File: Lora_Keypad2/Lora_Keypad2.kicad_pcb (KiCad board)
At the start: 2 copper layers, 53.3 x 76.2 mm, 7 parts, among them J1 OLED Conn

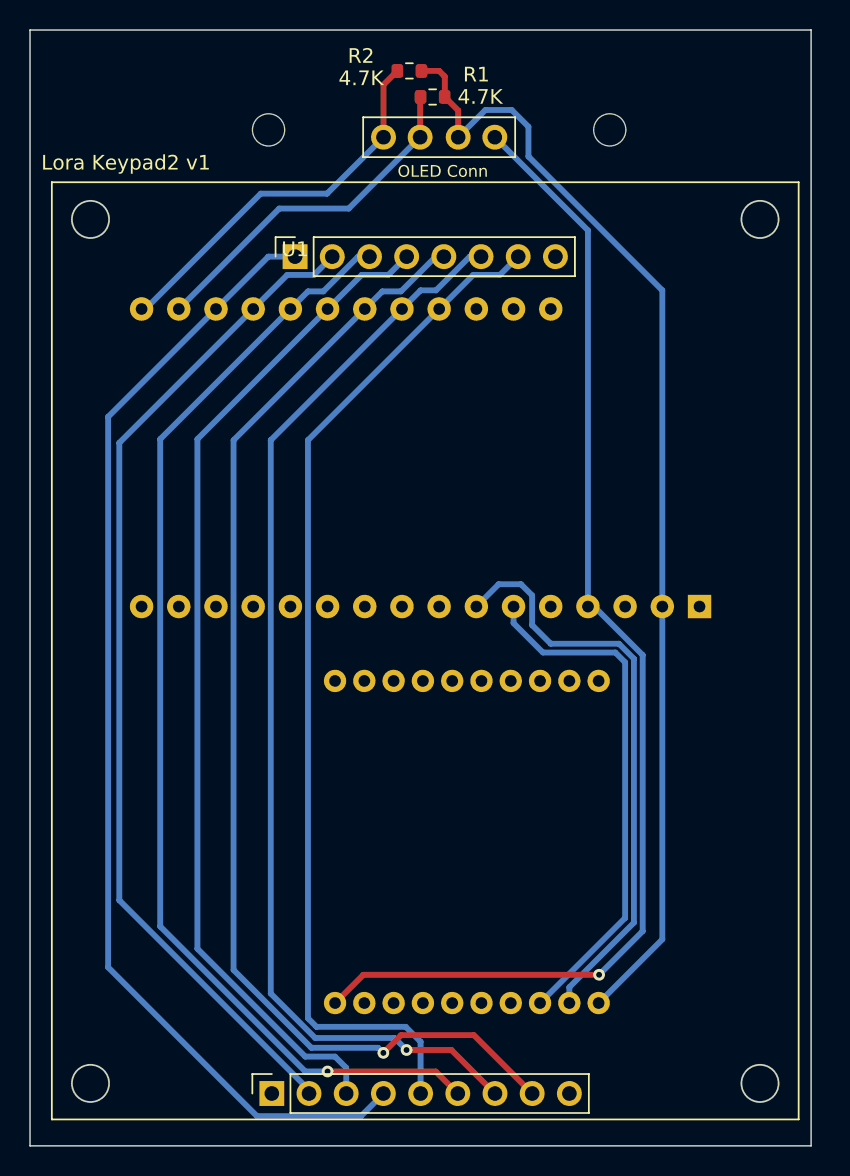
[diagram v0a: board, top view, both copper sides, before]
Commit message: update
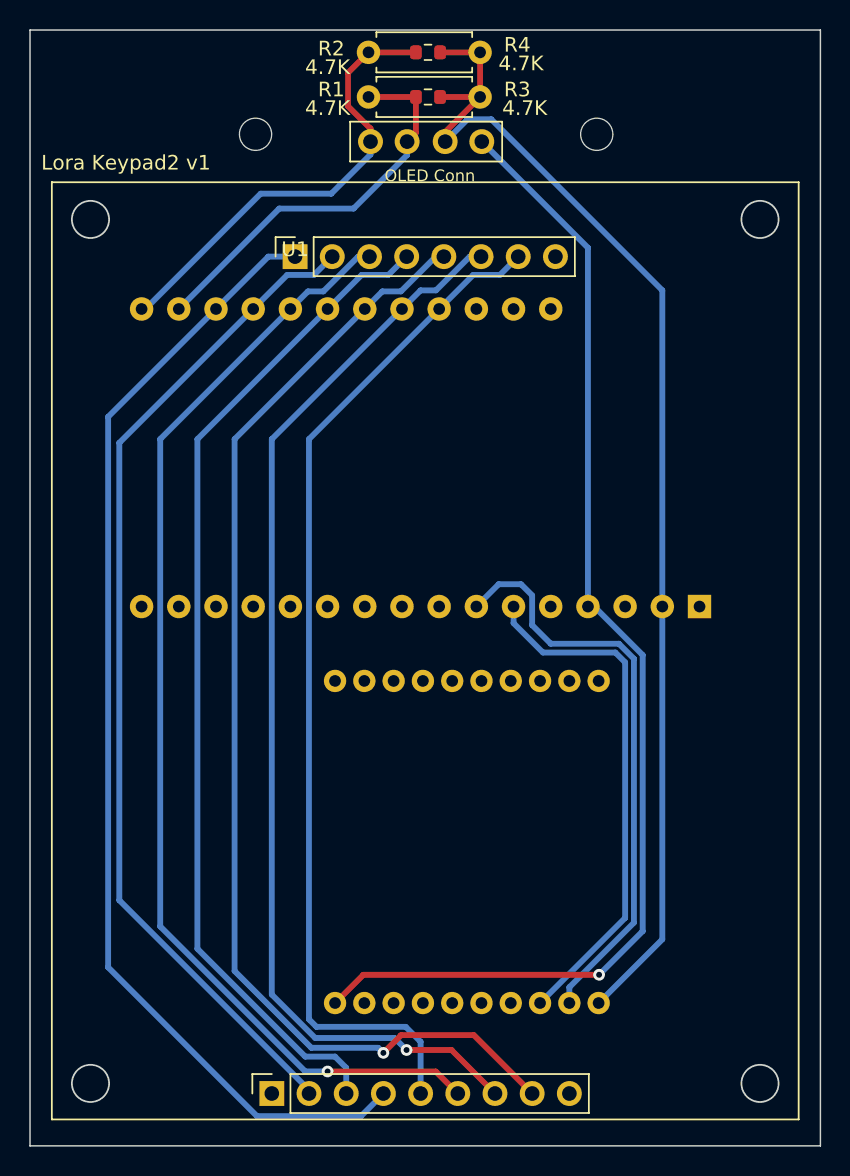
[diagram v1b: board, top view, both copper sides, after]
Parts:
- added R3: 4.7K, Resistor_THT:R_Axial_DIN0207_L6.3mm_D2.5mm_P7.62mm_Horizontal, F.Cu at (203.5, 60.5)
- added R4: 4.7K, Resistor_THT:R_Axial_DIN0207_L6.3mm_D2.5mm_P7.62mm_Horizontal, F.Cu at (203.5, 57.4)
- moved R2 1.80 mm to (199.9, 57.4)
- moved J1 0.94 mm to (199.8, 63.5)
- moved R1 0.32 mm to (199.9, 60.5)
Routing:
- net +3.3V: track 77.7 -> 83.3 mm
- net I2C_SDA: track 26.3 -> 31.4 mm
- net I2C_SCL: track 24.1 -> 27.4 mm
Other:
- board size 53.3 x 76.2 mm -> 54 x 76.2 mm
